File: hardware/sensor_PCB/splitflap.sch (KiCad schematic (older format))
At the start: 7 parts, among them J1 Conn_02x06_Odd_Even, J2 Conn_02x06_Odd_Even, J3 Screw_Terminal_01x04, J4 Screw_Terminal_01x04, J5 Screw_Terminal_01x04, J6 Screw_Terminal_01x04, J7 Conn_01x02_Male

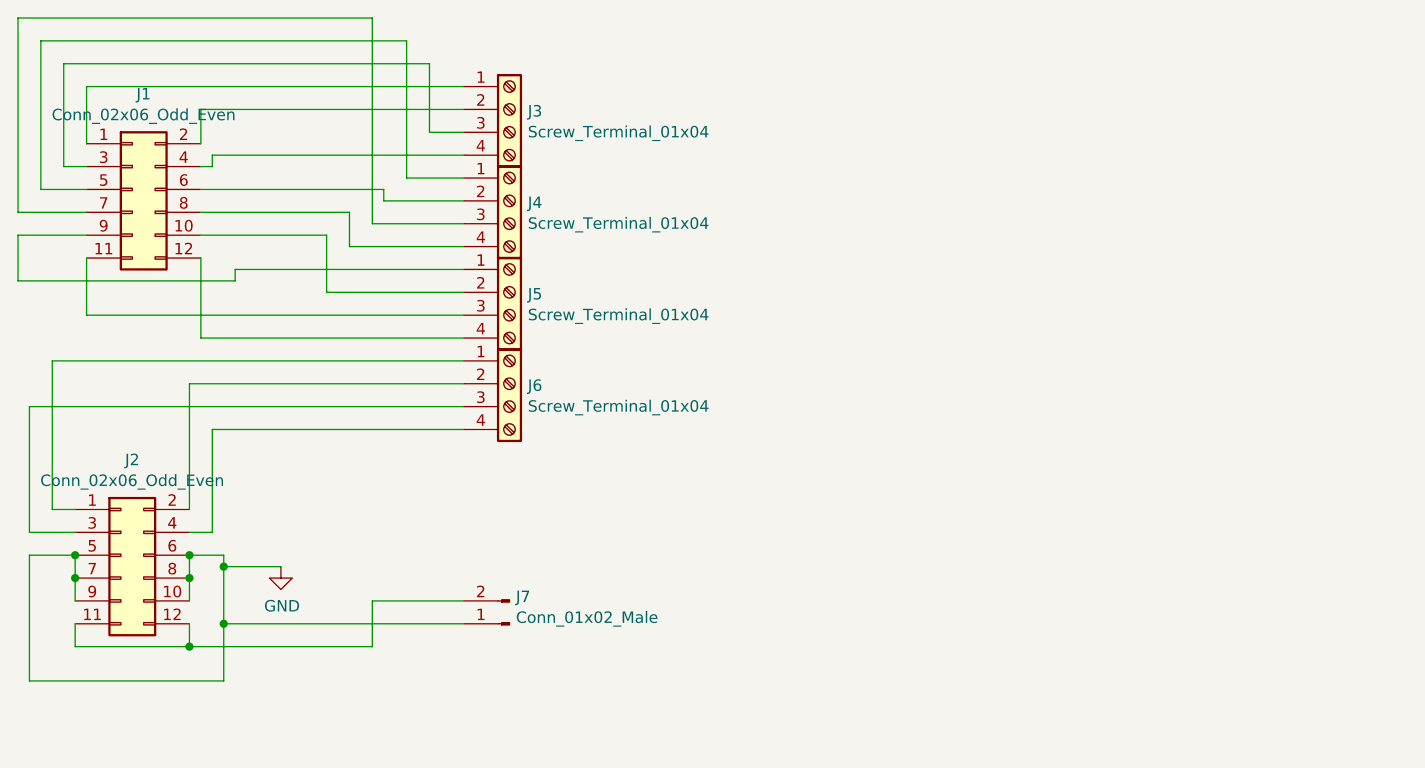
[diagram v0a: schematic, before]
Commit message: idk
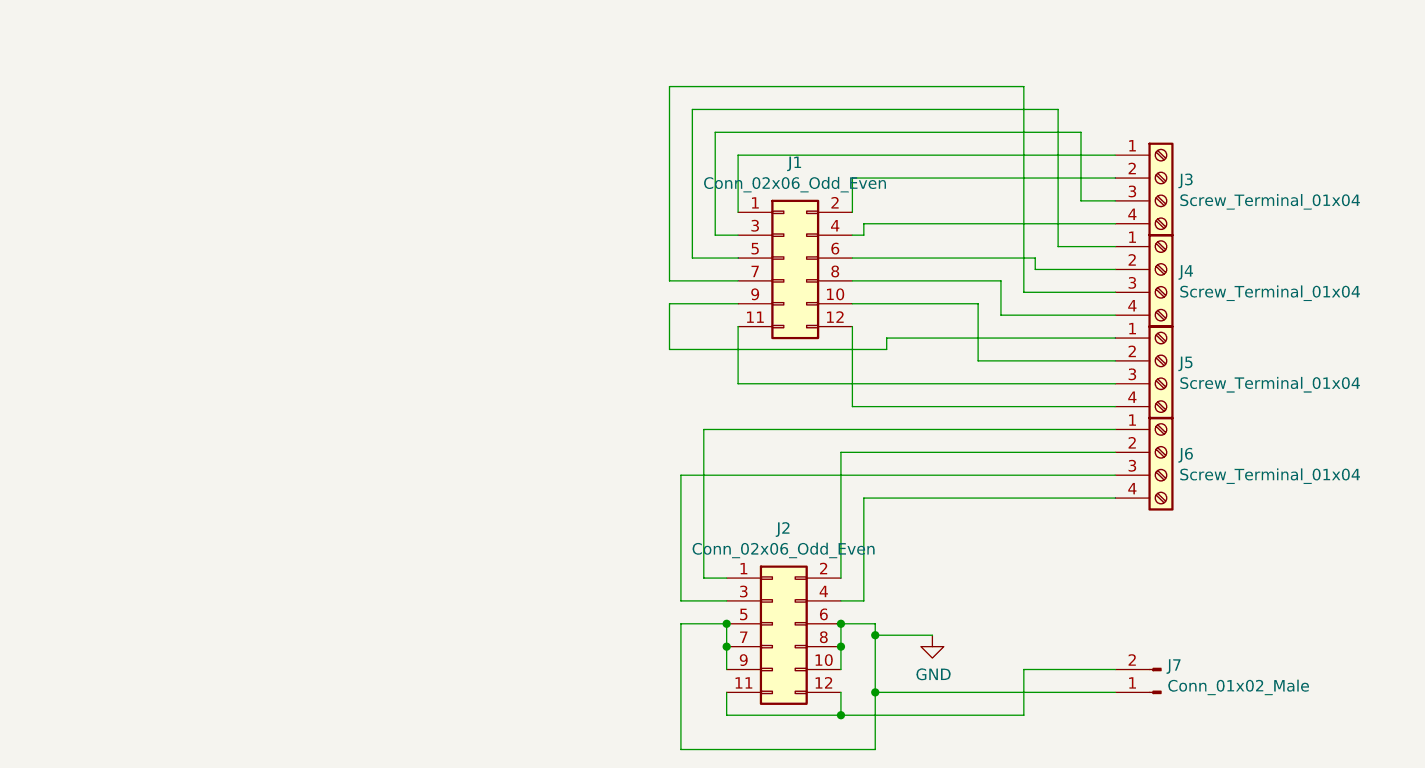
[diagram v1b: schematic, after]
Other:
- moved on the sheet: J1, J2, J3, J4, J5, J6, J7
